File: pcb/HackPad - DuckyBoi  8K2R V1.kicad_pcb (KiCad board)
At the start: 2 copper layers, 79.2 x 60.8 mm, 26 parts, among them SW1 RotaryEncoder_Switch, SW2 RotaryEncoder_Switch, SW3 SW_Push, SW4 SW_Push, SW5 SW_Push, SW6 SW_Push, SW7 SW_Push, SW8 SW_Push, SW9 SW_Push, U1 XIAO-RP2040-DIP

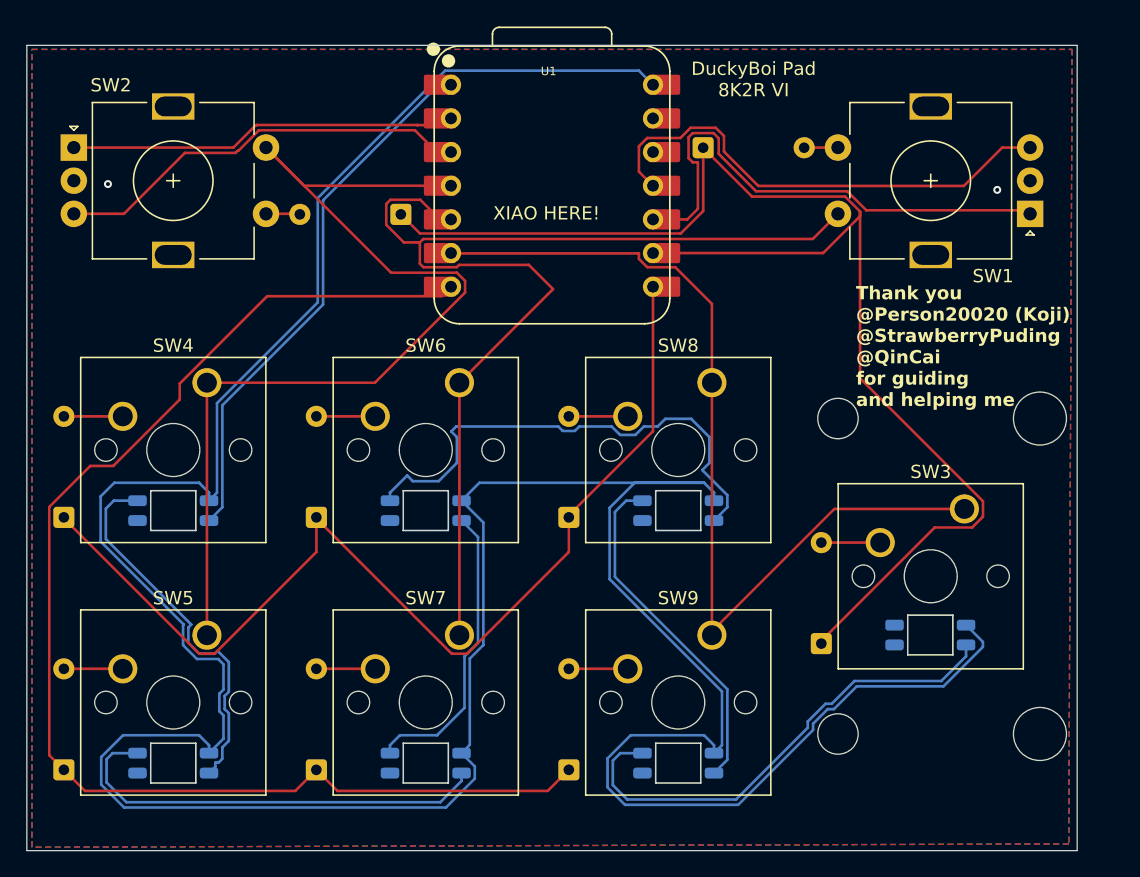
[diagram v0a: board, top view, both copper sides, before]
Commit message: update
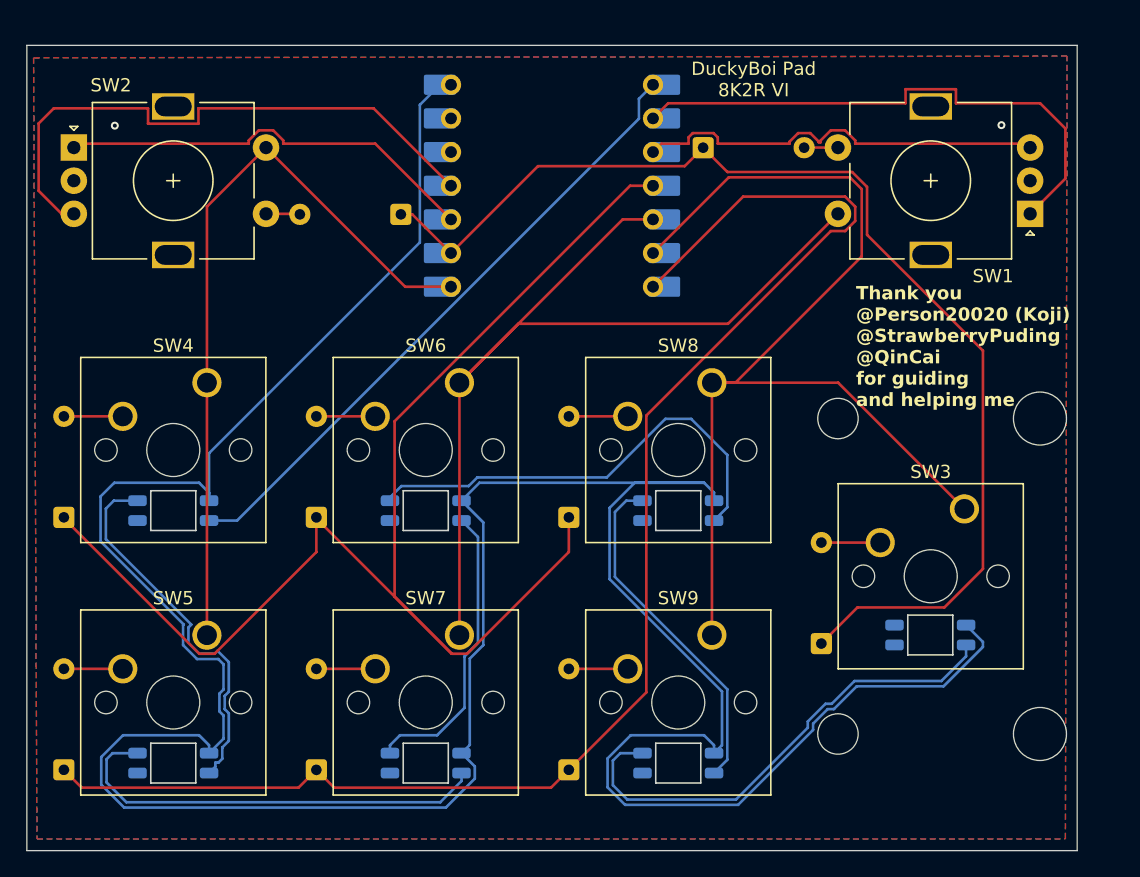
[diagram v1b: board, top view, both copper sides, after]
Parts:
- U1: moved to B.Cu
- turned U1 to 180 degrees
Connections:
- U1 pad 10: ROT2-A -> ROT1-A
- U1 pad 11: ROT2-B -> ROT1-B
- U1 pad 2: ROT1-A -> ROT2-A
- U1 pad 3: ROT1-B -> ROT2-B
- U1 pad 4: Col 0 -> Row 1
- U1 pad 8: Row 1 -> Col 0
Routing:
- net Row 1: track 78.3 -> 104.5 mm
- net Col 0: track 76.6 -> 56.9 mm
- net +5V: track 253.5 -> 236.2 mm
- net Row 0: track 104.0 -> 87.9 mm
- net ROT1-B: track 31.7 -> 44.8 mm
- net Row 2: track 98.9 -> 110.8 mm
- net Col 2: track 69.7 -> 80.9 mm
- net Col 1: track 83.5 -> 72.6 mm
- net Net-(D1-DIN): track 41.0 -> 48.0 mm
- net ROT2-B: track 37.2 -> 31.8 mm
- net ROT2-A: track 37.9 -> 42.0 mm
- net Net-(D4-DOUT): track 38.5 -> 34.6 mm
- net ROT1-A: track 29.4 -> 32.1 mm
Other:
- board text added: "XIAO HERE"
- board text removed: "XIAO HERE!"
